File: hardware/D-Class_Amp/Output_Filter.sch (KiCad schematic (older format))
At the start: 4 parts

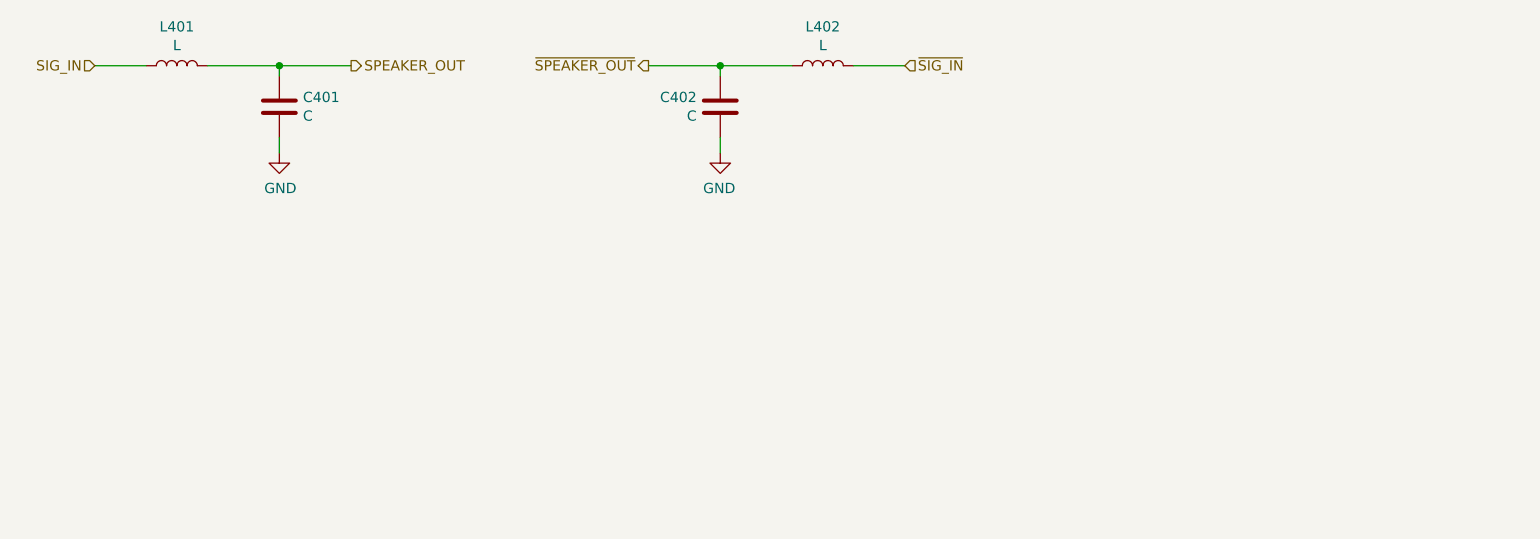
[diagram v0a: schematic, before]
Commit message: fixed remerge
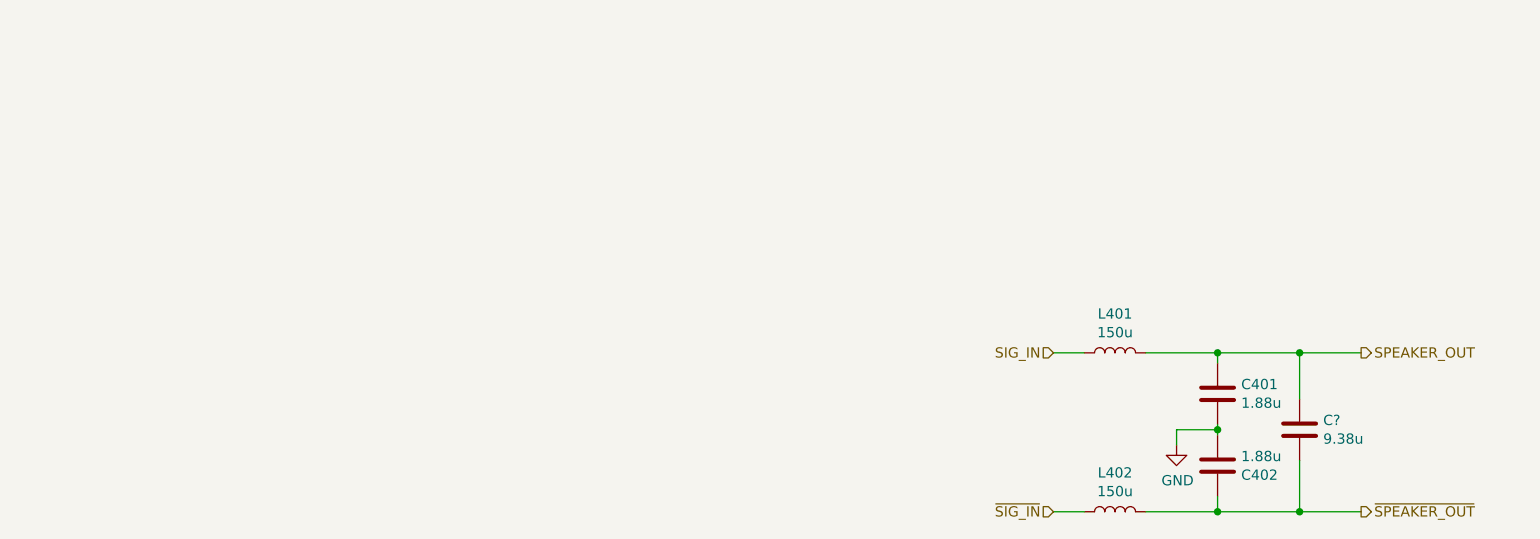
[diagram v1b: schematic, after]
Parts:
- added C?: 9.38u, symbol Device:C
- C401, C402: value C -> 1.88u
- L401, L402: value L -> 150u
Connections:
- net SPEAKER_OUT: now also C?.1
- net ~SIG_IN: now also L402.2; no longer L402.1
- net ~SPEAKER_OUT: now also L402.1, C?.2; no longer L402.2
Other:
- moved on the sheet: C401, C402, L401, L402
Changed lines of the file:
@@
 $Descr A4 11693 8268
 encoding utf-8
-Sheet 4 5
+Sheet 1 1
 Title ""
 Date ""
@@
 Comment4 ""
 $EndDescr
-Text HLabel 3700 3500 0    50   Input ~ 0
+Text HLabel 8375 4900 0    50   Input ~ 0
 SIG_IN
-Text HLabel 7650 3500 2    50   Input ~ 0
+Text HLabel 8375 5675 0    50   Input ~ 0
 ~SIG_IN
 $Comp
 L Device:L L401
 U 1 1 61193FAD
-P 4100 3500
-F 0 "L401" V 4290 3500 50  0000 C CNN
-F 1 "L" V 4199 3500 50  0000 C CNN
-F 2 "" H 4100 3500 50  0001 C CNN
-F 3 "~" H 4100 3500 50  0001 C CNN
-	1    4100 3500
+P 8675 4900
+F 0 "L401" V 8865 4900 50  0000 C CNN
+F 1 "150u" V 8774 4900 50  0000 C CNN
+F 2 "" H 8675 4900 50  0001 C CNN
+F 3 "~" H 8675 4900 50  0001 C CNN
+	1    8675 4900
 	0    -1   -1   0
 $EndComp
@@
 L Device:L L402
 U 1 1 61195264
-P 7250 3500
-F 0 "L402" V 7440 3500 50  0000 C CNN
-F 1 "L" V 7349 3500 50  0000 C CNN
-F 2 "" H 7250 3500 50  0001 C CNN
-F 3 "~" H 7250 3500 50  0001 C CNN
-	1    7250 3500
+P 8675 5675
+F 0 "L402" V 8865 5675 50  0000 C CNN
+F 1 "150u" V 8774 5675 50  0000 C CNN
+F 2 "" H 8675 5675 50  0001 C CNN
+F 3 "~" H 8675 5675 50  0001 C CNN
+	1    8675 5675
 	0    1    -1   0
 $EndComp
@@
 L Device:C C401
 U 1 1 611955B4
-P 4600 3700
-F 0 "C401" H 4715 3746 50  0000 L CNN
-F 1 "C" H 4715 3655 50  0000 L CNN
-F 2 "" H 4638 3550 50  0001 C CNN
-F 3 "~" H 4600 3700 50  0001 C CNN
-	1    4600 3700
+P 9175 5100
+F 0 "C401" H 9290 5146 50  0000 L CNN
+F 1 "1.88u" H 9290 5055 50  0000 L CNN
+F 2 "" H 9213 4950 50  0001 C CNN
+F 3 "~" H 9175 5100 50  0001 C CNN
+	1    9175 5100
 	1    0    0    -1
 $EndComp
@@
 L Device:C C402
 U 1 1 61195DF7
-P 6750 3700
-F 0 "C402" H 6865 3746 50  0000 L CNN
-F 1 "C" H 6865 3655 50  0000 L CNN
-F 2 "" H 6788 3550 50  0001 C CNN
-F 3 "~" H 6750 3700 50  0001 C CNN
-	1    6750 3700
-	-1   0    0    -1
+P 9175 5450
+F 0 "C402" H 9290 5496 50  0000 L CNN
+F 1 "1.88u" H 9290 5405 50  0000 L CNN
+F 2 "" H 9213 5300 50  0001 C CNN
+F 3 "~" H 9175 5450 50  0001 C CNN
+	1    9175 5450
+	1    0    0    1
 $EndComp
 Wire Wire Line
-	3700 3500 3950 3500
+	8375 4900 8525 4900
 Wire Wire Line
-	4250 3500 4600 3500
+	8825 4900 9175 4900
 Wire Wire Line
-	4600 3500 4600 3550
+	9175 4900 9175 4950
 Wire Wire Line
-	4600 3500 4950 3500
-Connection ~ 4600 3500
+	9175 4900 9575 4900
+Connection ~ 9175 4900
 Wire Wire Line
-	7650 3500 7400 3500
+	8375 5675 8525 5675
 Wire Wire Line
-	7100 3500 6750 3500
+	8825 5675 9175 5675
 Wire Wire Line
-	6750 3500 6750 3550
+	9175 5675 9175 5600
 Wire Wire Line
-	6750 3500 6400 3500
-Connection ~ 6750 3500
+	9175 5675 9575 5675
+Connection ~ 9175 5675
 $Comp
 L power:GND #PWR0401
 U 1 1 611D879A
-P 4600 3925
-F 0 "#PWR0401" H 4600 3675 50  0001 C CNN
-F 1 "GND" H 4605 3752 50  0000 C CNN
-F 2 "" H 4600 3925 50  0001 C CNN
-F 3 "" H 4600 3925 50  0001 C CNN
-	1    4600 3925
+P 8975 5350
+F 0 "#PWR0401" H 8975 5100 50  0001 C CNN
+F 1 "GND" H 8980 5177 50  0000 C CNN
+F 2 "" H 8975 5350 50  0001 C CNN
+F 3 "" H 8975 5350 50  0001 C CNN
+	1    8975 5350
 	1    0    0    -1
 $EndComp
+Wire Wire Line
+	9175 5300 9175 5275
+Text HLabel 9875 4900 2    50   Output ~ 0
+SPEAKER_OUT
+Text HLabel 9875 5675 2    50   Output ~ 0
+~SPEAKER_OUT
+Wire Wire Line
+	9175 5275 8975 5275
+Wire Wire Line
+	8975 5275 8975 5350
+Connection ~ 9175 5275
+Wire Wire Line
+	9175 5275 9175 5250
+Connection ~ 9575 5675
+Wire Wire Line
+	9575 5675 9875 5675
+Connection ~ 9575 4900
+Wire Wire Line
+	9575 4900 9875 4900
+Wire Wire Line
+	9575 5425 9575 5675
+Wire Wire Line
+	9575 5125 9575 4900
 $Comp
-L power:GND #PWR0402
-U 1 1 611D8B24
-P 6750 3925
-F 0 "#PWR0402" H 6750 3675 50  0001 C CNN
-F 1 "GND" H 6755 3752 50  0000 C CNN
-F 2 "" H 6750 3925 50  0001 C CNN
-F 3 "" H 6750 3925 50  0001 C CNN
-	1    6750 3925
-	-1   0    0    -1
+L Device:C C?
+U 1 1 611BA813
+P 9575 5275
+F 0 "C?" H 9690 5321 50  0000 L CNN
+F 1 "9.38u" H 9690 5230 50  0000 L CNN
+F 2 "" H 9613 5125 50  0001 C CNN
+F 3 "~" H 9575 5275 50  0001 C CNN
+	1    9575 5275
+	1    0    0    -1
 $EndComp
-Wire Wire Line
-	6750 3925 6750 3850
-Wire Wire Line
-	4600 3925 4600 3850
-Text HLabel 4950 3500 2    50   Output ~ 0
-SPEAKER_OUT
-Text HLabel 6400 3500 0    50   Output ~ 0
-~SPEAKER_OUT
 $EndSCHEMATC
